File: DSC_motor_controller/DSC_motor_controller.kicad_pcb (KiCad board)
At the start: 4 copper layers, 105.9 x 99.3 mm, 102 parts, among them P1 PH_A, P2 PH_B, P3 PH_C, P4 SUPPLY, P5 GND, Q1 IRFS7730TRLPBF, Q2 IRFS7730TRLPBF, Q3 IRFS7730TRLPBF, Q4 IRFS7730TRLPBF, Q5 IRFS7730TRLPBF, Q6 IRFS7730TRLPBF

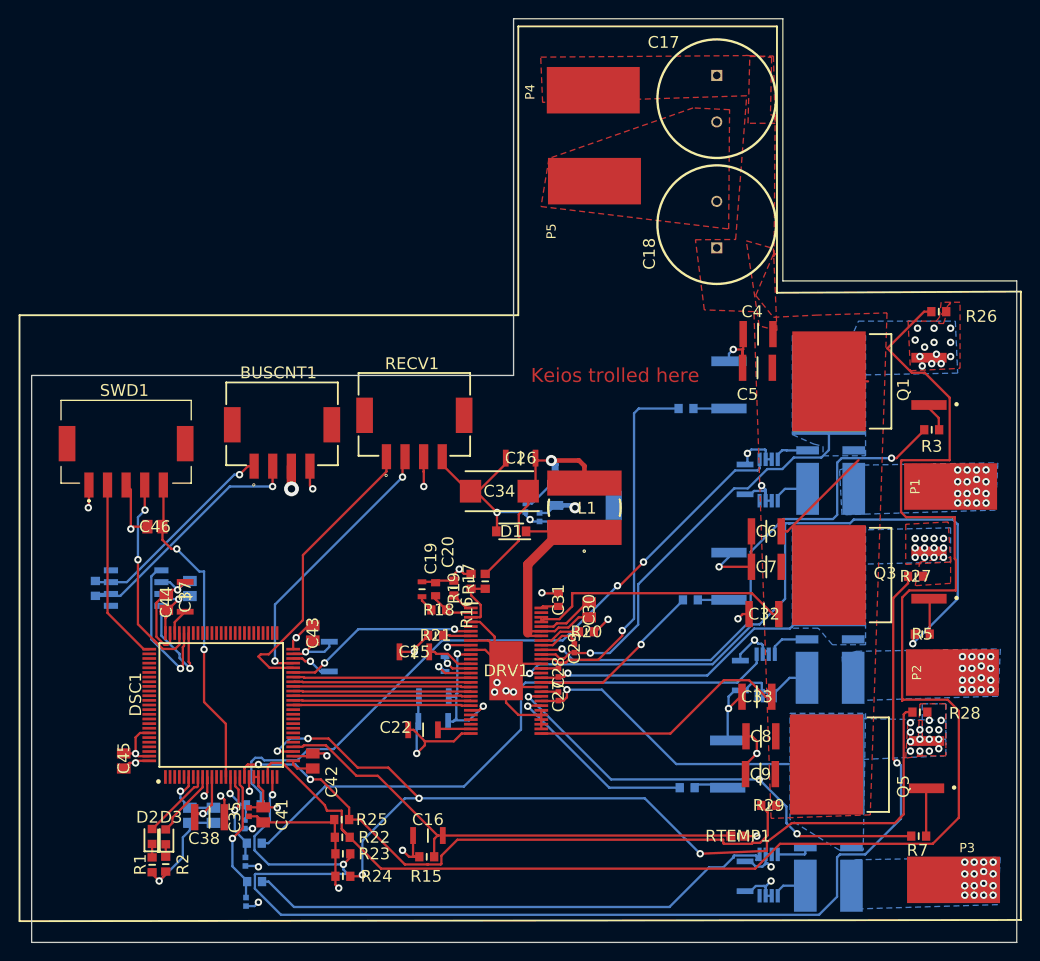
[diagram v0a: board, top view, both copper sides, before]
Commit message: PCB version that will be given to Eric's friend for review
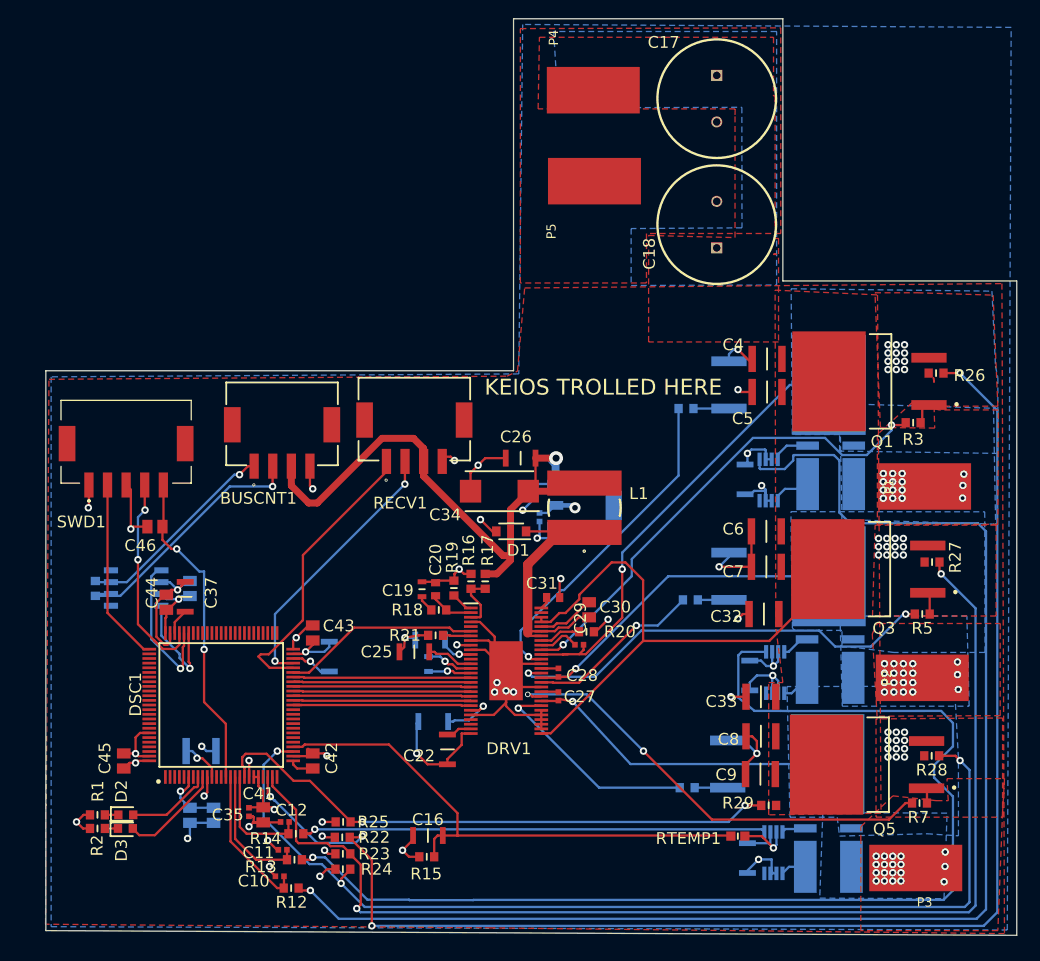
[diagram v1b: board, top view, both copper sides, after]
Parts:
- C10, C11, C12, R12, R13, R14: moved to F.Cu
- C38: moved to B.Cu
- moved R12 9.83 mm to (84.5, 191.8)
- moved C12 9.55 mm to (83.9, 184.7), turned to 180 degrees
- moved R2 8.28 mm to (63.7, 185.4), turned to 0 degrees
- moved R1 7.96 mm to (63.7, 183.9), turned to 0 degrees
- moved C38 7.17 mm to (74.9, 177.0)
- moved R14 6.79 mm to (85.1, 185.9)
- moved C10 6.73 mm to (83.3, 190.5), turned to 180 degrees
- moved R26 6.61 mm to (153.9, 136.4), turned to 180 degrees
- moved C24 6.11 mm to (99.5, 165.1)
- moved R28 4.87 mm to (153.4, 177.5), turned to 180 degrees
- moved R13 4.67 mm to (84.9, 188.7)
- moved D3 4.43 mm to (66.7, 185.4), turned to 0 degrees
- moved P3 4.26 mm to (151.7, 189.6)
- moved C11 4.20 mm to (83.6, 187.7), turned to 180 degrees
- moved D2 3.66 mm to (66.8, 183.9), turned to 0 degrees
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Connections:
- C24 pad 1: Net-(C23-Pad1) -> Net-(C24-Pad1)
- DRV1 pad 11: Net-(C23-Pad1) -> Net-(C24-Pad1)
- DRV1 pad 24: Net-(DRV1-Pad24) -> GND
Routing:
- net /Power/C_A: track 74.0 -> 149.3 mm, vias 2 -> 1
- net /Power/C_B: track 64.9 -> 124.0 mm, vias 0 -> 1
- net +5V: track 35.2 -> 70.1 mm, vias 3 -> 1
- net /Motor_Driver/GH_B: track 75.2 -> 47.3 mm
- net GND: track 217.7 -> 205.4 mm, vias 32 -> 41
- net SUPPLY: track 72.6 -> 60.7 mm
- net /Motor_Driver/Volt_A: track 167.1 -> 155.7 mm, vias 0 -> 4
- net /Motor_Driver/Volt_B: track 137.7 -> 126.4 mm, vias 3 -> 2
- net /Motor_controller/Curr_A: track 5.69 -> 16.0 mm, vias 1 -> 0
- net Net-(C23-Pad1): track 16.2 -> 6.55 mm, vias 2 -> 1
- net /Motor_Driver/Volt_C: track 102.3 -> 109.7 mm, vias 5 -> 3
- net /Motor_Driver/GH_A: track 59.6 -> 52.2 mm
- net /Power/C_C: track 57.6 -> 50.6 mm, vias 0 -> 1
- net /Motor_Driver/Batt_voltage: track 68.7 -> 62.0 mm
- net /Motor_controller/Curr_B: track 9.56 -> 14.5 mm, vias 1 -> 0
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- added copper zone on B.Cu, net GND
- added copper zone on F.Cu, net Net-(P1-Pad1)
- added copper zone on F.Cu, net Net-(P2-Pad1)
- added copper zone on F.Cu, net Net-(P3-Pad1)
- added copper zone on B.Cu, net SUPPLY
- removed copper zone on In1.Cu, net +5V
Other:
- board size 105.9 x 99.3 mm -> 104.4 x 98.6 mm
- rule via_min_size: 0.4 -> 0
- board text added: "KEIOS TROLLED HERE"
- board text removed: "Keios trolled here"
